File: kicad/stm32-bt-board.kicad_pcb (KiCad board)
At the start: 4 copper layers, 55 x 35.2 mm, 54 parts, among them J1 1909763-1, J2 2171790001, J3 Conn_ARM_SWD_TagConnect_TC2030, J4 S4B-PH-K-S(LF)(SN), Q1 S9013-E, SW1 B3U-1000P, SW2 B3U-1000P, U1 MIC5365-3.3YD5, U2 USBLC6-2SC6, U3 USBLC6-2SC6, U4 STM32WB55CEU6, X1 32MHz, X2 32kHz768

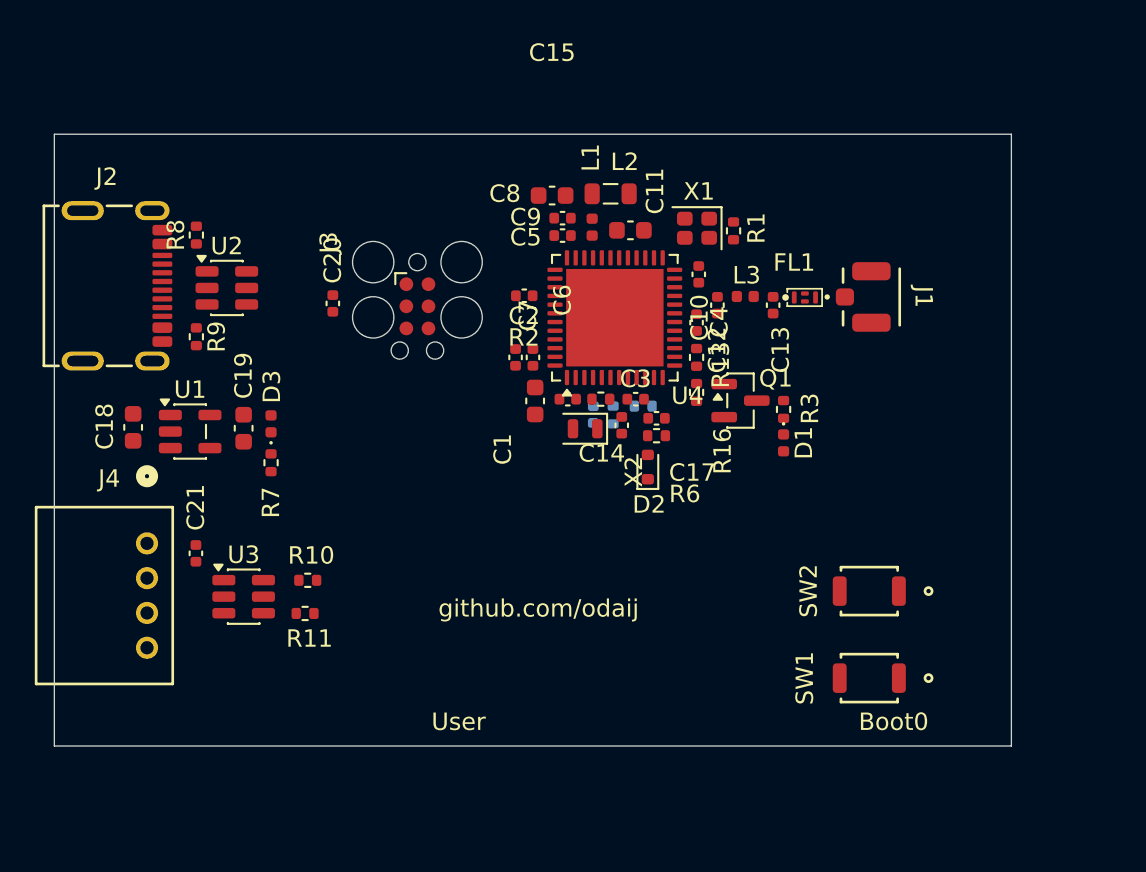
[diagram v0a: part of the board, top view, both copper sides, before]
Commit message: i am in a hurry
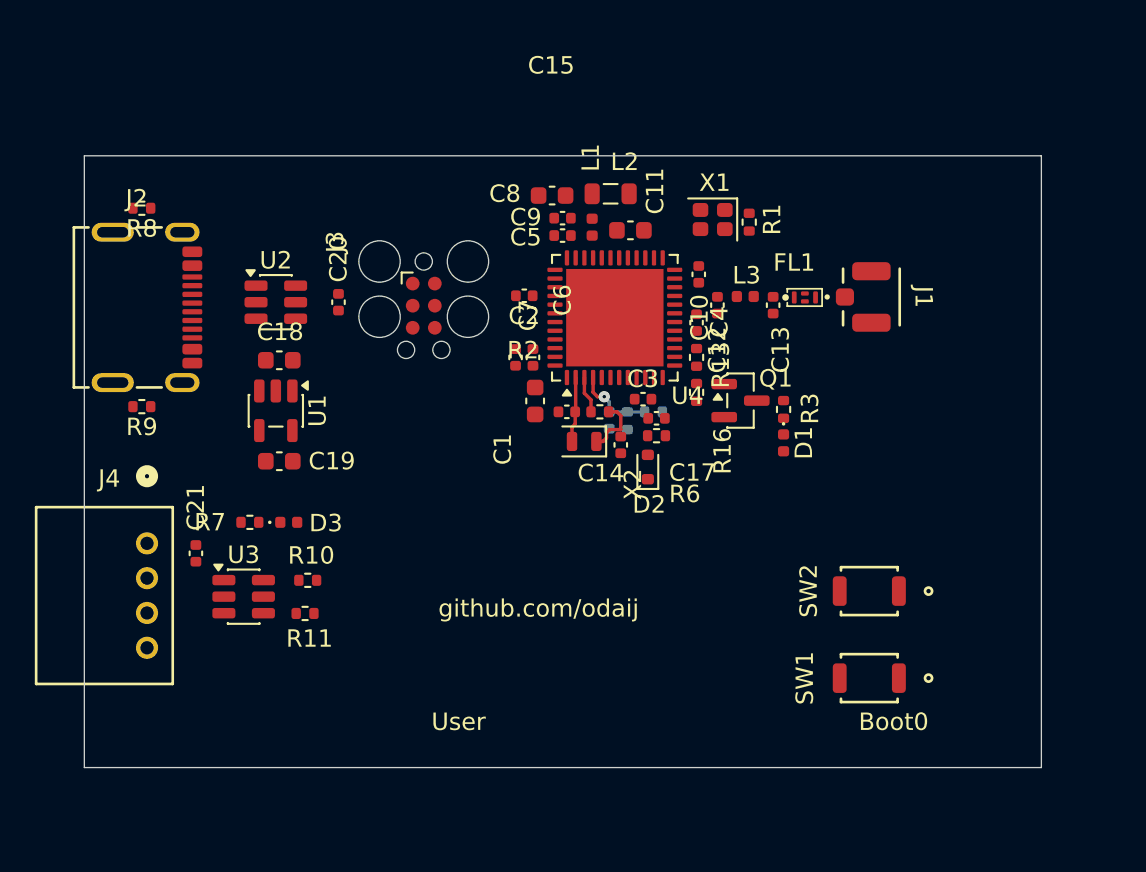
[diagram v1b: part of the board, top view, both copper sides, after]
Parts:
- moved C18 9.24 mm to (135.1, 99.7), turned to 180 degrees
- moved D3 5.75 mm to (135.6, 109.0), turned to 0 degrees
- moved R9 5.09 mm to (127.2, 102.4), turned to 180 degrees
- moved U1 5.07 mm to (134.9, 102.6), turned to -90 degrees
- moved R7 3.63 mm to (133.4, 109.0), turned to 180 degrees
- moved R8 3.49 mm to (127.2, 91.0), turned to 180 degrees
- moved U2 2.93 mm to (134.9, 96.4)
- moved C19 2.79 mm to (135.1, 105.5), turned to 180 degrees
- moved J2 2.12 mm to (126.8, 96.7)
- moved C14 1.13 mm to (154.7, 104.6)
- moved R1 1.03 mm to (162.1, 91.8)
- moved X1 1.03 mm to (160.0, 91.7)
- moved C16 0.97 mm to (154.1, 103.2)
- moved R5 0.88 mm to (155.1, 103.2)
- moved C15 0.73 mm to (151.6, 102.7)
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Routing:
- net /Microcontroller/BOOT0: track 0.00 -> 4.62 mm, vias 0 -> 1
- net /Microcontroller/OSC_LSE_IN: track 0.00 -> 3.76 mm
- net /Microcontroller/Crystals/OSC_LSE_OUT_R: track 0.00 -> 3.44 mm
- net /Microcontroller/OSC_LSE_OUT: track 0.00 -> 2.13 mm
